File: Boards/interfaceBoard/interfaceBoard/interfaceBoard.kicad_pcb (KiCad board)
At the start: 2 copper layers, 100 x 100 mm, 34 parts, among them J1 12V input (molex), J2 Barrel_Jack_Switch, J3 Interface With Arduino, J4 Conn_02x17_Odd_Even, J5 DaisyCainOut, J6 Conn_02x17_Odd_Even, SW1 SW_SPDT, U1 74HC595, U10 74HC595, U11 TBD62783A, U12 74HC165, U2 TBD62783A, U3 74HC165, U4 74HC595, U5 TBD62783A, U6 74HC165, U7 74HC595, U8 TBD62783A, U9 74HC165

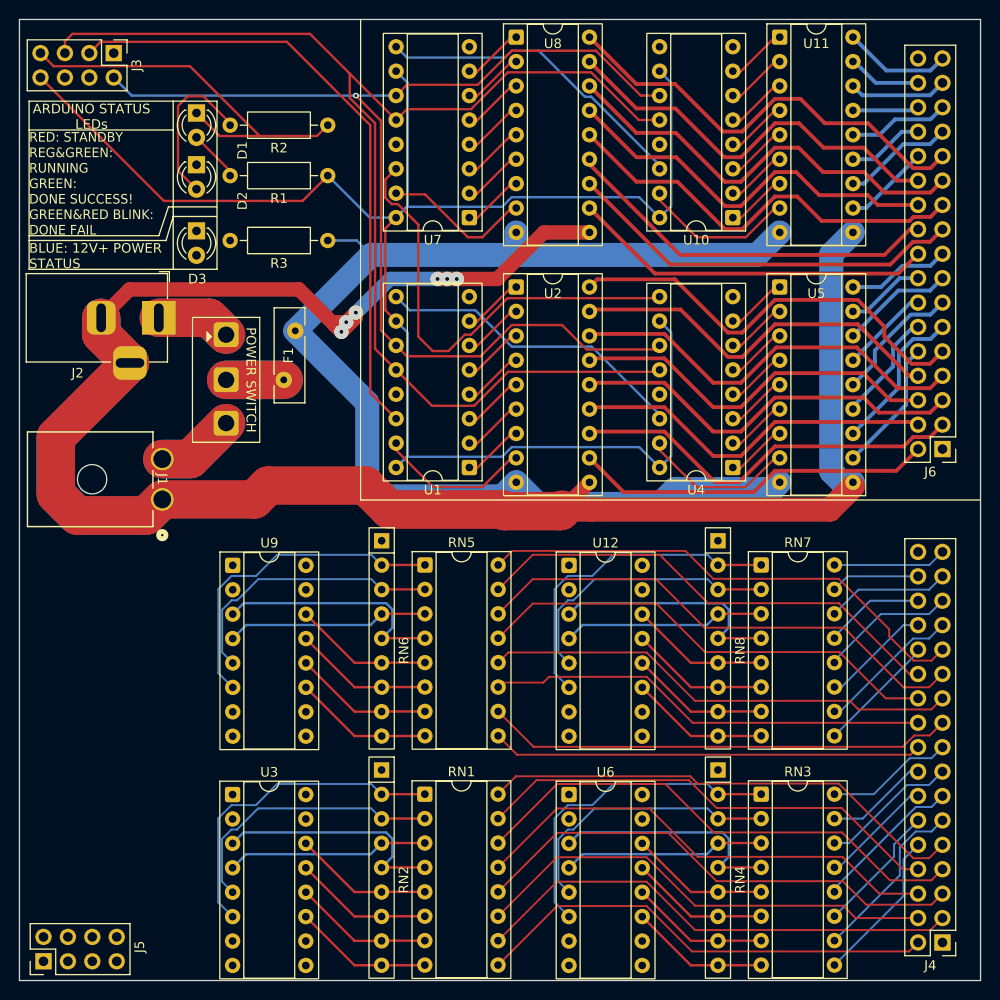
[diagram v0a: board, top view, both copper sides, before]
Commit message: DRC PASSED
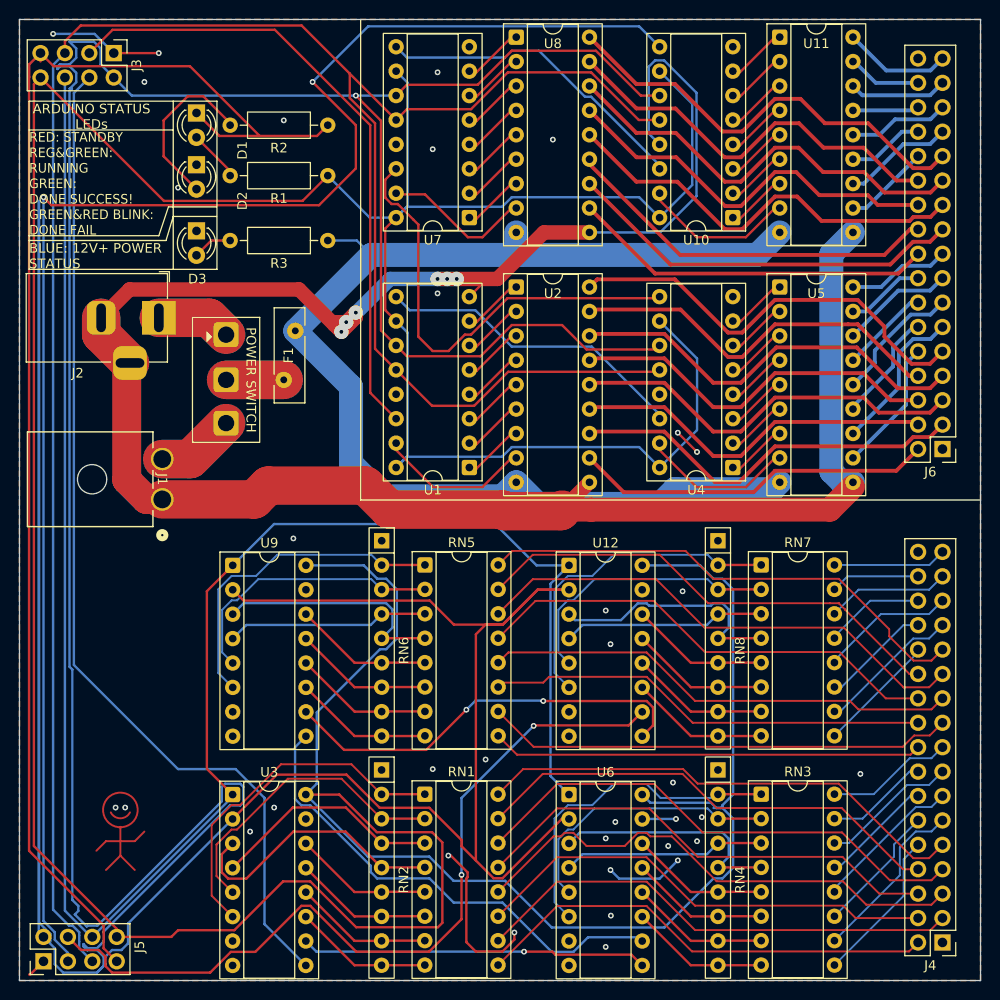
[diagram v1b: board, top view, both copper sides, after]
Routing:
- net CLK: track 119.6 -> 579.9 mm
- net 5V+: track 180.2 -> 479.6 mm
- net LOAD: track 0.00 -> 201.6 mm
- net /MOSI_sheet3/QH': track 0.00 -> 165.2 mm, vias 0 -> 2
- net /MISO: track 0.00 -> 106.6 mm
- net /STATUS: track 41.5 -> 141.1 mm
- net LATCH: track 134.6 -> 232.2 mm
- net /MISO_sheet3/SerIn: track 0.00 -> 84.4 mm, vias 0 -> 2
- net GND: track 243.9 -> 305.9 mm, vias 6 -> 41
- net /MISO_sheet1/SerIn: track 0.00 -> 50.9 mm
- net /MISO_sheet2/SerIn: track 0.00 -> 43.6 mm, vias 0 -> 2
- net /MISO_sheet/SerIn: track 0.00 -> 36.1 mm, vias 0 -> 1
- net Net-(D3-A): track 0.00 -> 4.14 mm
- net Net-(RN1-R4.1): track 25.4 -> 28.5 mm
- net Net-(RN1-R3.1): track 21.1 -> 24.1 mm
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- added copper zone on B.Cu, net GND
- added copper zone on F.Cu, net GND
